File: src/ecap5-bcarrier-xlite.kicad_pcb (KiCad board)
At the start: 4 copper layers, 161.3 x 55.2 mm, 55 parts, among them J1 DDR4_SODIMM_Board, J2 DDR4_SODIMM_Board, J3 Conn_01x04, J4 Conn_01x04, J5 USB_C_Receptacle_USB2.0_14P, J6 Conn_Coaxial, J7 Conn_Coaxial, J8 Conn_Coaxial, J9 1935161, Q1 BC846BR13, Q2 BC846BR13, SW1 RESET_SOM1, SW2 RESET_SOM2, SW3 USER1, SW4 USER1, U1 FT232RN, U2 AP7375-33SA-7

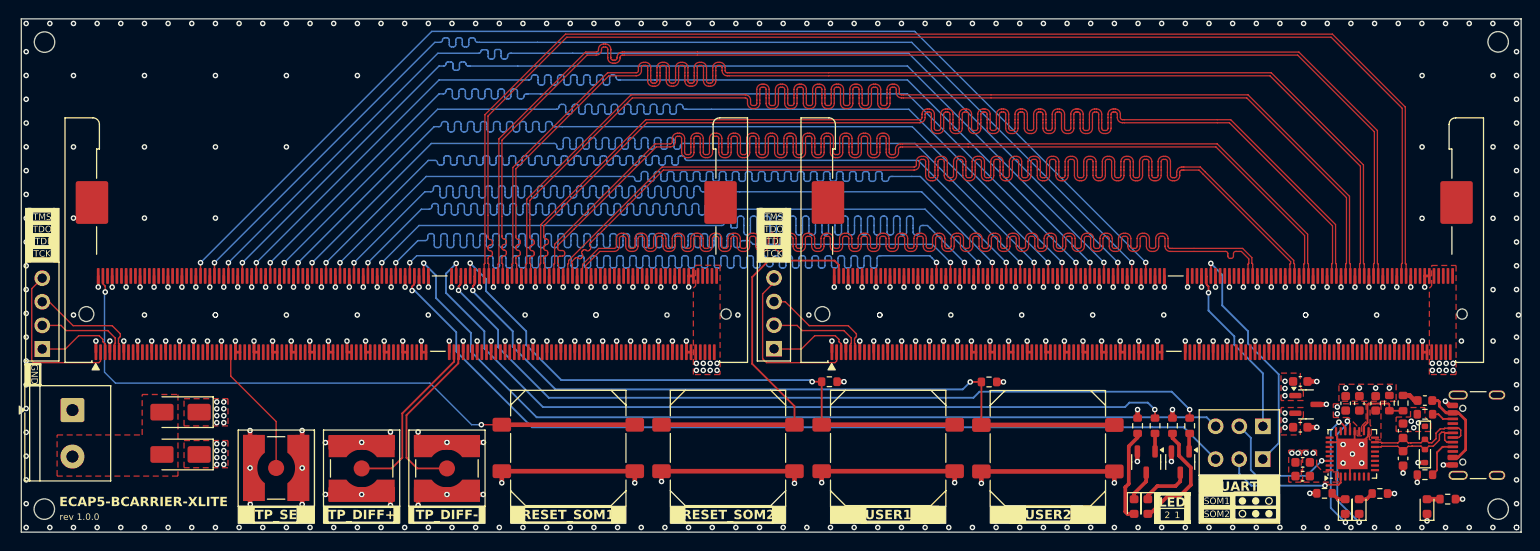
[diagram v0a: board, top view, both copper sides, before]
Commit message: Fix erc issues
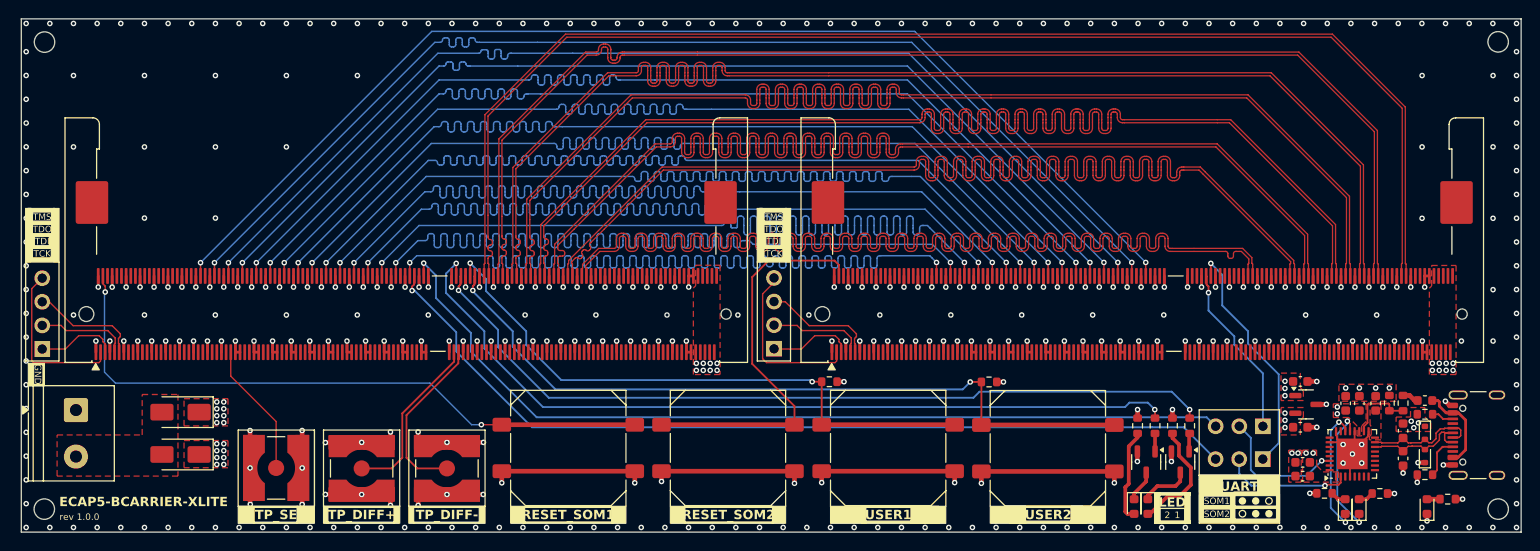
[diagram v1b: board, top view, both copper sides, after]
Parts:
- moved J9 0.38 mm to (36.8, 105.1)
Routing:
- net GND: vias 433 -> 427
